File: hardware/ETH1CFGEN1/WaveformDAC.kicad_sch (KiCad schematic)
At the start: 128 parts, among them K301 G6SU-2F-DC3, K302 G6SU-2F-DC3, Q301 MMBT5087LT1G, U301 TL072CDT, U302 AD9744, U303 LT1016CS8, U304 THS3001IDG, X1 SG5032CAN 50.000000M-TJGA3

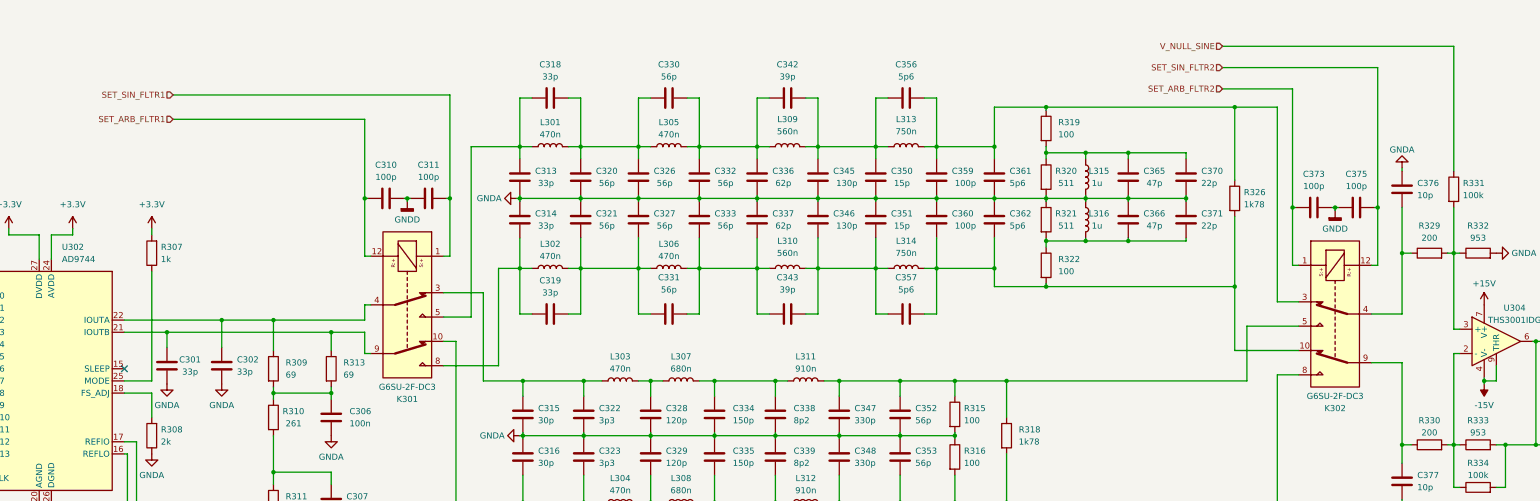
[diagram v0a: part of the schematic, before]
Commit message: PCB design
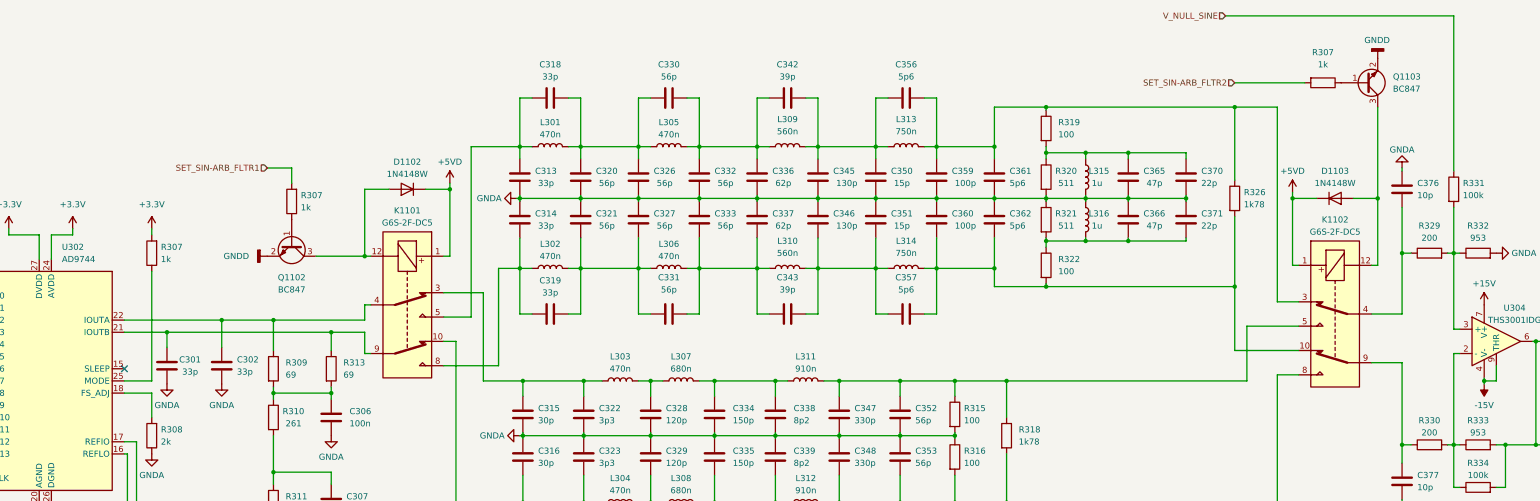
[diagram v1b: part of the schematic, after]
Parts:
- removed C310, C311, C373, C375: 100p, Capacitor_SMD:C_0603_1608Metric_Pad1.08x0.95mm_HandSolder, symbol Device:C
- removed K301, K302: G6SU-2F-DC3, Relay_SMD:Relay_DPDT_Omron_G6SK-2F, symbol Relay:G6SU-2
- added D1102, D1103: 1N4148W, Diode_SMD:D_SOD-123, symbol Diode:1N4148W
- added K1101, K1102: G6S-2F-DC5, Relay_SMD:Relay_DPDT_Omron_G6SK-2F, symbol Relay:G6S-2
- added Q1102, Q1103: BC847, Package_TO_SOT_SMD:SOT-23, symbol Transistor_BJT:BC847
- added R307 (x2): 1k, Resistor_SMD:R_0603_1608Metric_Pad0.98x0.95mm_HandSolder, symbol Device:R
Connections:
- net GNDD: now also Q1102.2 (E), Q1103.2 (E)
- net at C301.1, R313.1, U302.21 (IOUTB): now also K1101.9
- net at C302.1, R309.1, U302.22 (IOUTA): now also K1101.4
- net at C377.1, R330.1: now also K1102.9
- net at C347.1, C352.1, L311.2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: now also K1102.5
- net at C315.1, C322.1, L303.1: now also K1101.3
- net at C356.2, C359.1, C361.1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: now also K1102.3
- net at C316.2, C323.2, L304.1: now also K1101.10
- net at C348.2, C353.2, L312.2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: now also K1102.8
- net at C357.2, C360.2, C362.2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: now also K1102.10
- net at C313.1, C318.1, L301.1: now also K1101.5
- net at C376.2, R329.1: now also K1102.4
- net at C314.2, C319.1, L302.1: now also K1101.8
- new net: Q1103.1 (B), R307.1
- new net: D1103.2 (A), K1102.12, Q1103.3 (C)
- new net: D1102.2 (A), K1101.12, Q1102.3 (C)
- new net: Q1102.1 (B), R307.1
- new net +5VD: D1102.1 (K), D1103.1 (K), K1101.1, K1102.1
- new net SET_SIN-ARB_FLTR1: R307.2
- new net SET_SIN-ARB_FLTR2: R307.2
